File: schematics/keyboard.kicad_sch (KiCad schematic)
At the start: 32 parts, among them J2 Mini-DIN-6, Q1 2N7000, Q2 2N7000, Q3 2N7000, Q4 2N7000, Q5 2N7000, U18 74HC14, U19 74HC04, U21 ATF22V10C-7, U22 74HC280, U23 74HC165, U24 74HC595, U25 74HC165, U26 74HC595, U37 74HC245

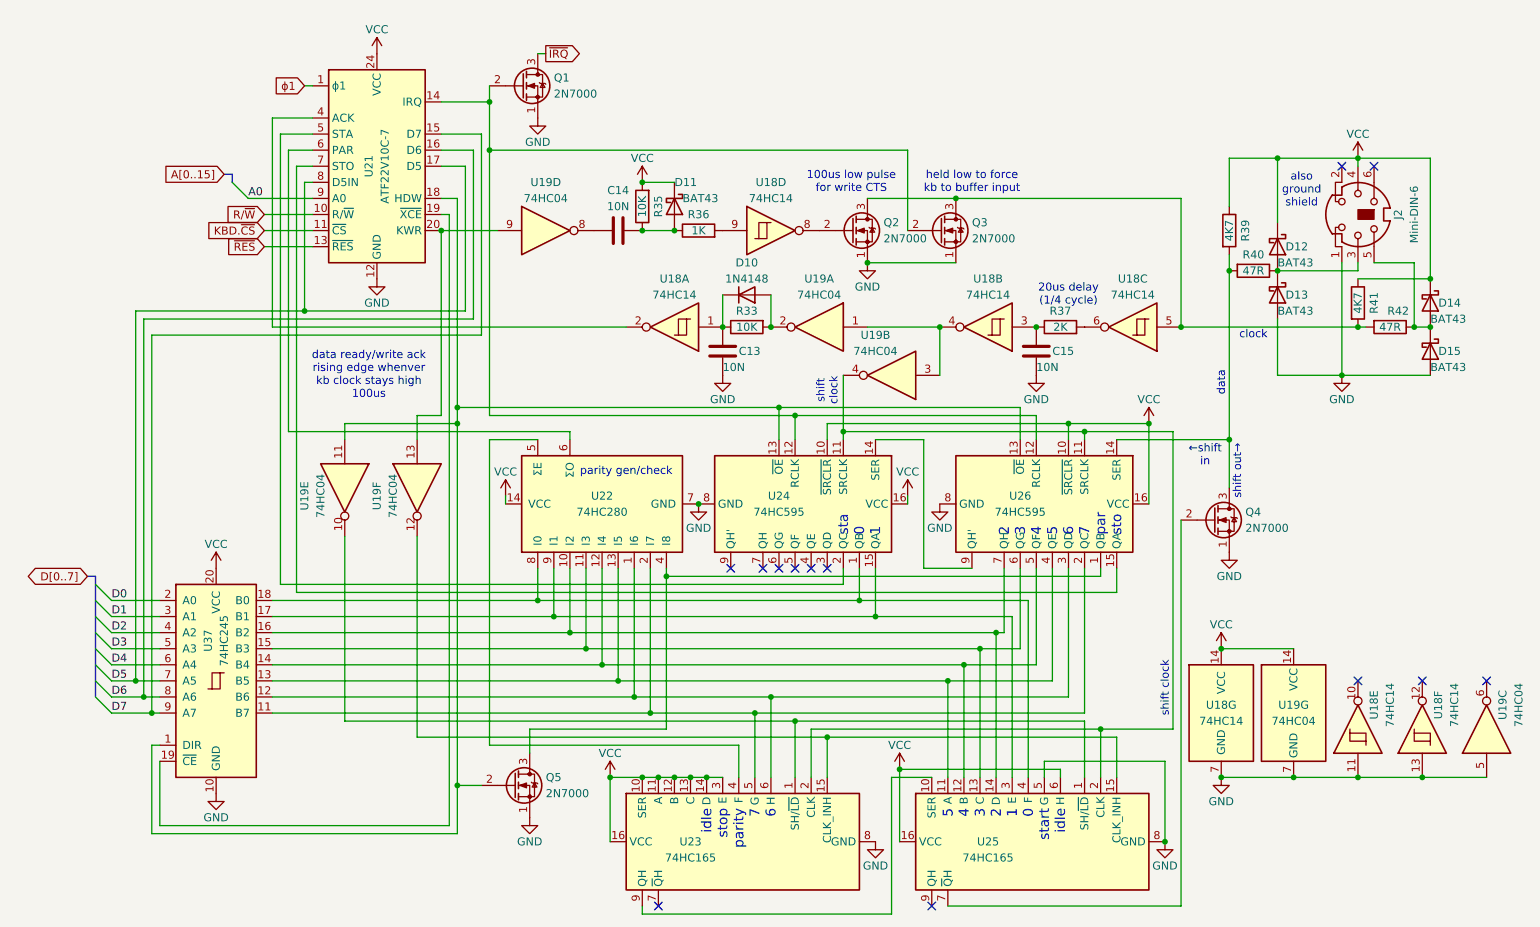
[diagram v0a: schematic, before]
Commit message: keyboard output debug--still WIP
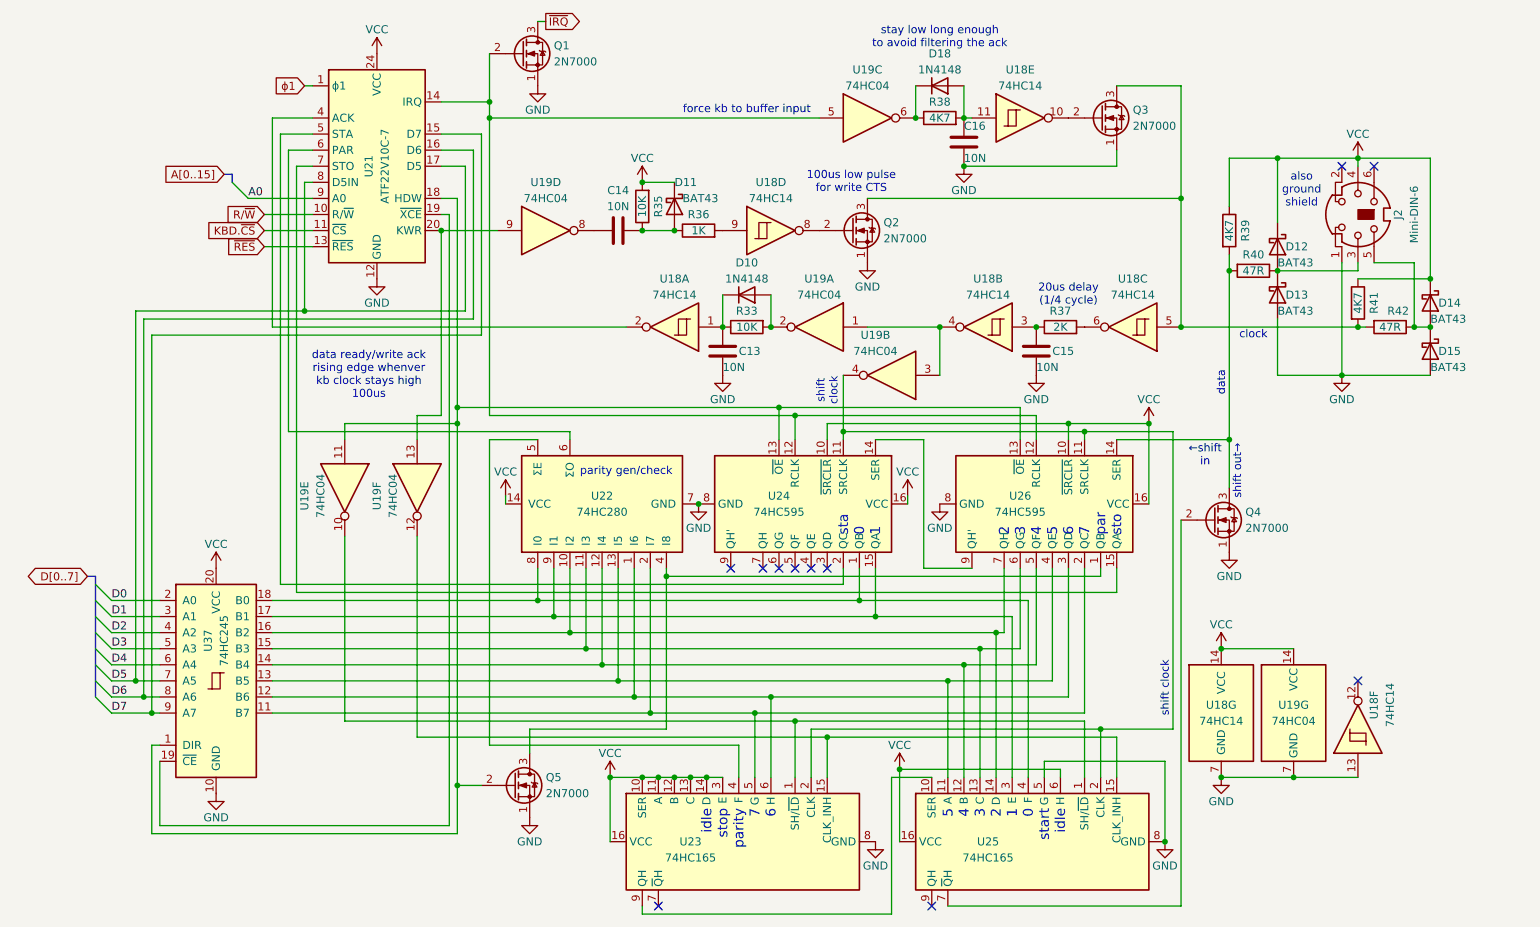
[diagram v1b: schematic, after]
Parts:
- added C16: 10N, symbol Device:C
- added D18: 1N4148, Diode_THT:D_DO-35_SOD27_P7.62mm_Horizontal, symbol Diode:1N4148
- added R38: 4K7, symbol Device:R
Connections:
- net GND: now also U18.13, C16.2; no longer U18.11, U18.13, U19.5
- net at Q1.2 (G), U21.14 (IRQ), U24.12 (RCLK)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: now also U19.5; no longer Q3.2 (G)
- net at U19.6: now also D18.1 (K), R38.1
- new net: Q3.2 (G), U18.10
- new net: C16.1, D18.2 (A), R38.2, U18.11
- no-connect marks 13 -> 11
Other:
- note added: "force kb to buffer input"
- note added: "stay low long enough to avoid filtering the ack"
- note removed: "held low to force kb to buffer input"
- moved on the sheet: Q1, Q3, U18E, U19C
